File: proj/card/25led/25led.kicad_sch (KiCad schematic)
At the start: 41 parts, among them U1 ATtiny404-SS

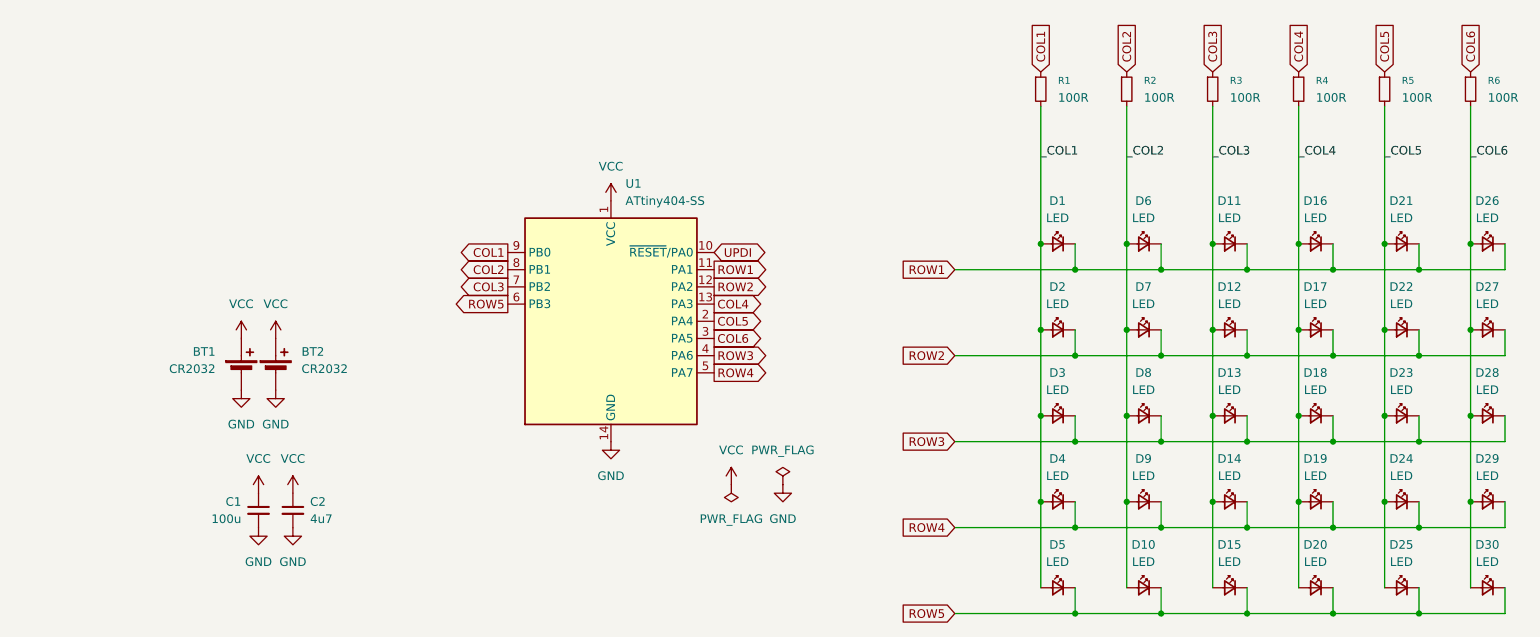
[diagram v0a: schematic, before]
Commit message: -
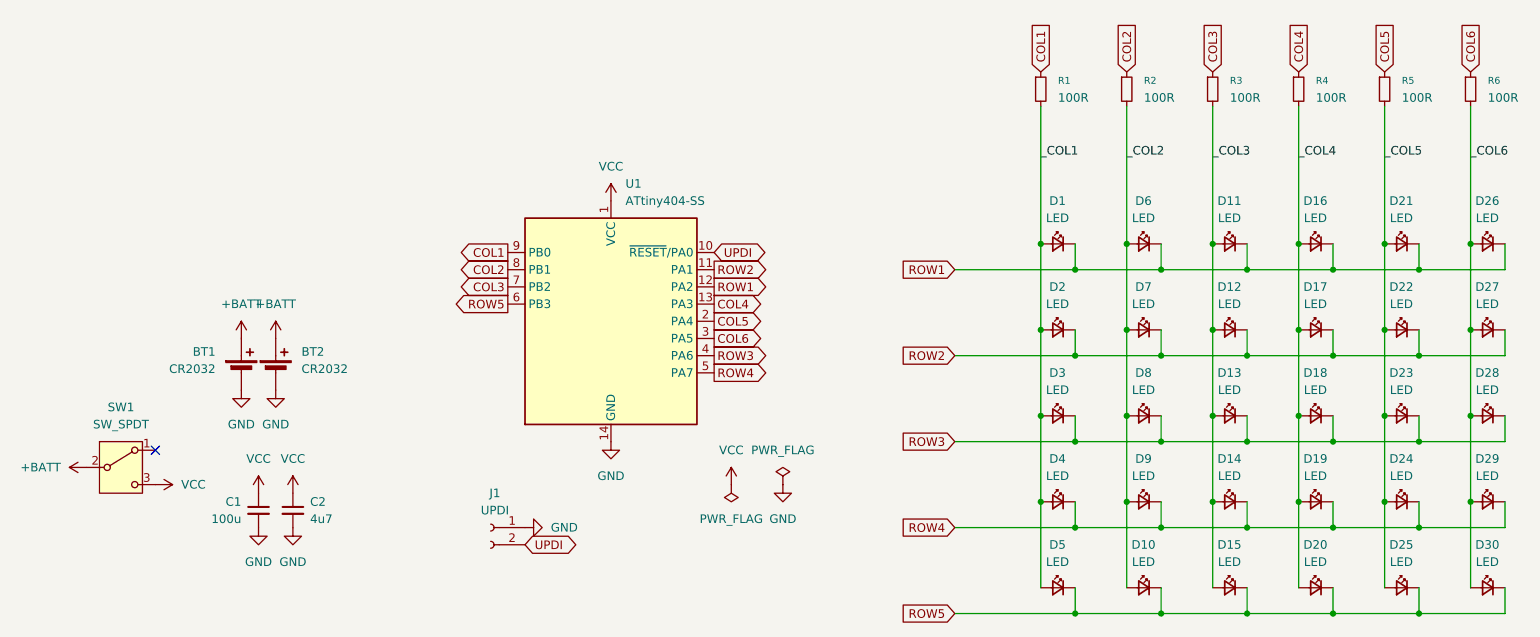
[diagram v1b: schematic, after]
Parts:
- added J1: UPDI, Connector_PinSocket_2.54mm:PinSocket_1x02_P2.54mm_Vertical, symbol Connector:Conn_01x02_Socket
- added SW1: SW_SPDT, Button_Switch_THT:SW_Slide_SPDT_Straight_CK_OS102011MS2Q, symbol Switch:SW_SPDT
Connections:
- net GND: now also J1.1 (Pin_1)
- net ROW1: now also U1.12 (PA2); no longer U1.11 (PA1)
- net ROW2: now also U1.11 (PA1); no longer U1.12 (PA2)
- net UPDI: now also J1.2 (Pin_2)
- net VCC: now also SW1.3 (C); no longer BT1.1 (+), BT2.1 (+)
- new net +BATT: BT1.1 (+), BT2.1 (+), SW1.2 (B)
- no-connect marks 0 -> 1
